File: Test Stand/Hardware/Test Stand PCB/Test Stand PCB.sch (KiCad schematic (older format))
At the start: 18 parts, among them J1 Screw_Terminal_01x02, J2 Screw_Terminal_01x02, J3 Screw_Terminal_01x02, J4 Screw_Terminal_01x04, J5 Screw_Terminal_01x02, U1 AdafruitHuzzah32Breakout, U2 Adafruit_MAX31856, U3 Adafruit_MAX31856, U4 Adafruit_MAX31856, U5 Adafruit_MAX31856, U7 INA_122P, U8 Adafruit_MicroSD_Breakout

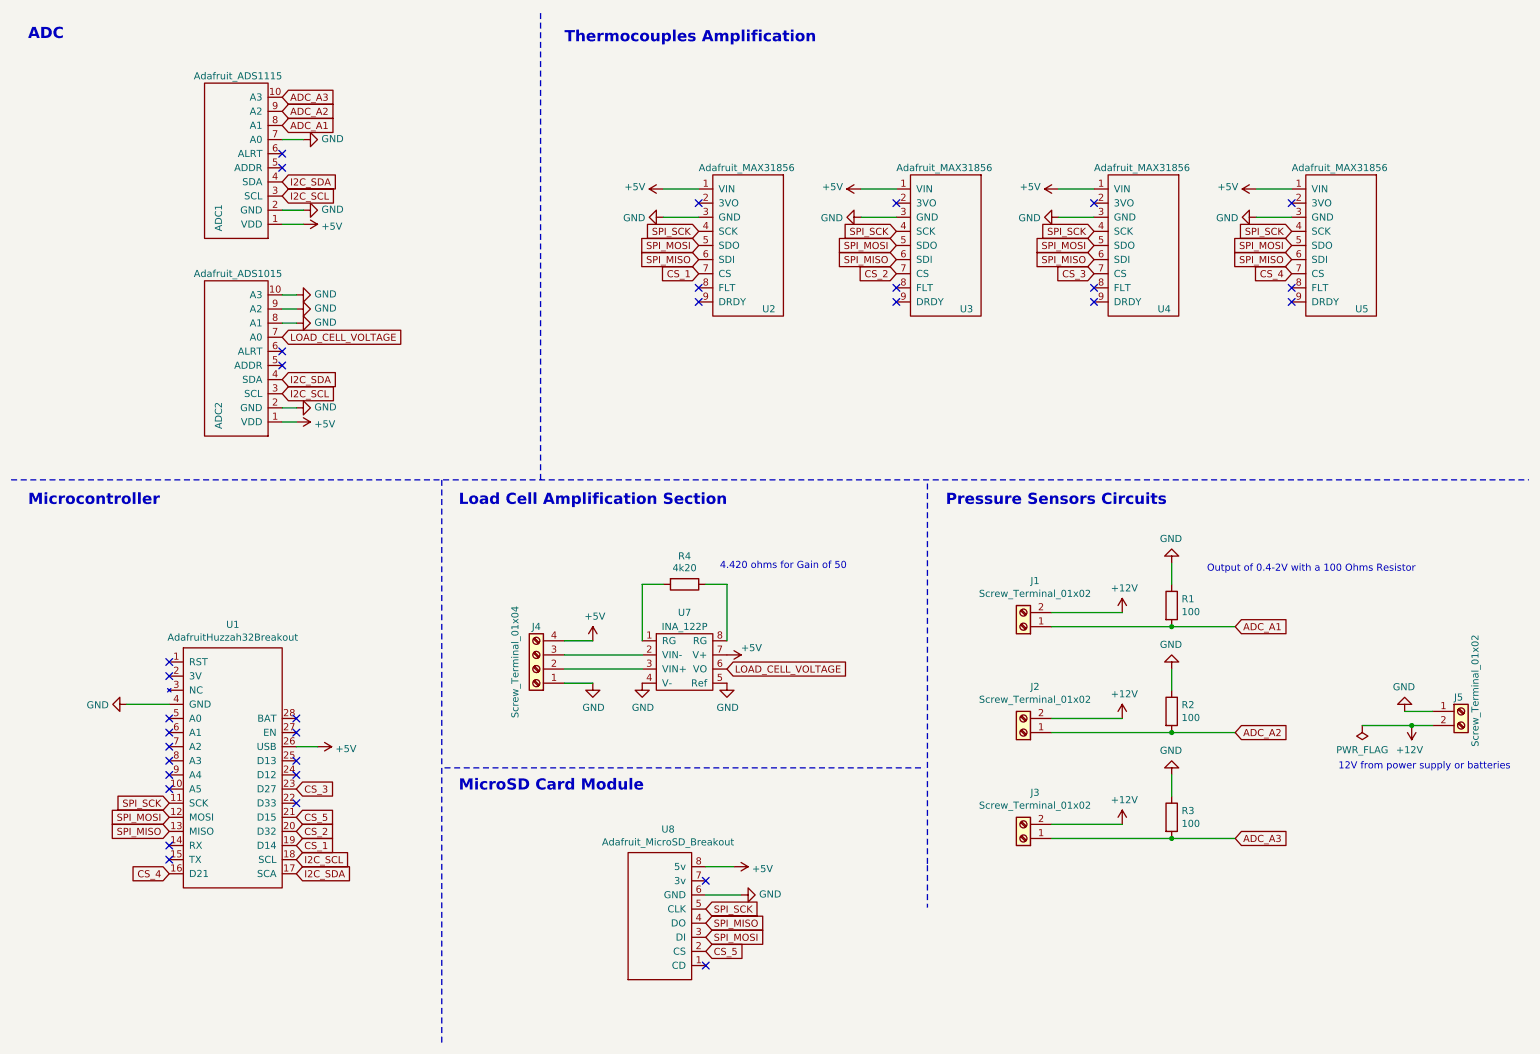
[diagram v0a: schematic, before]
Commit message: Added gerber file for manufacturing of Test Stand PCB v1.0
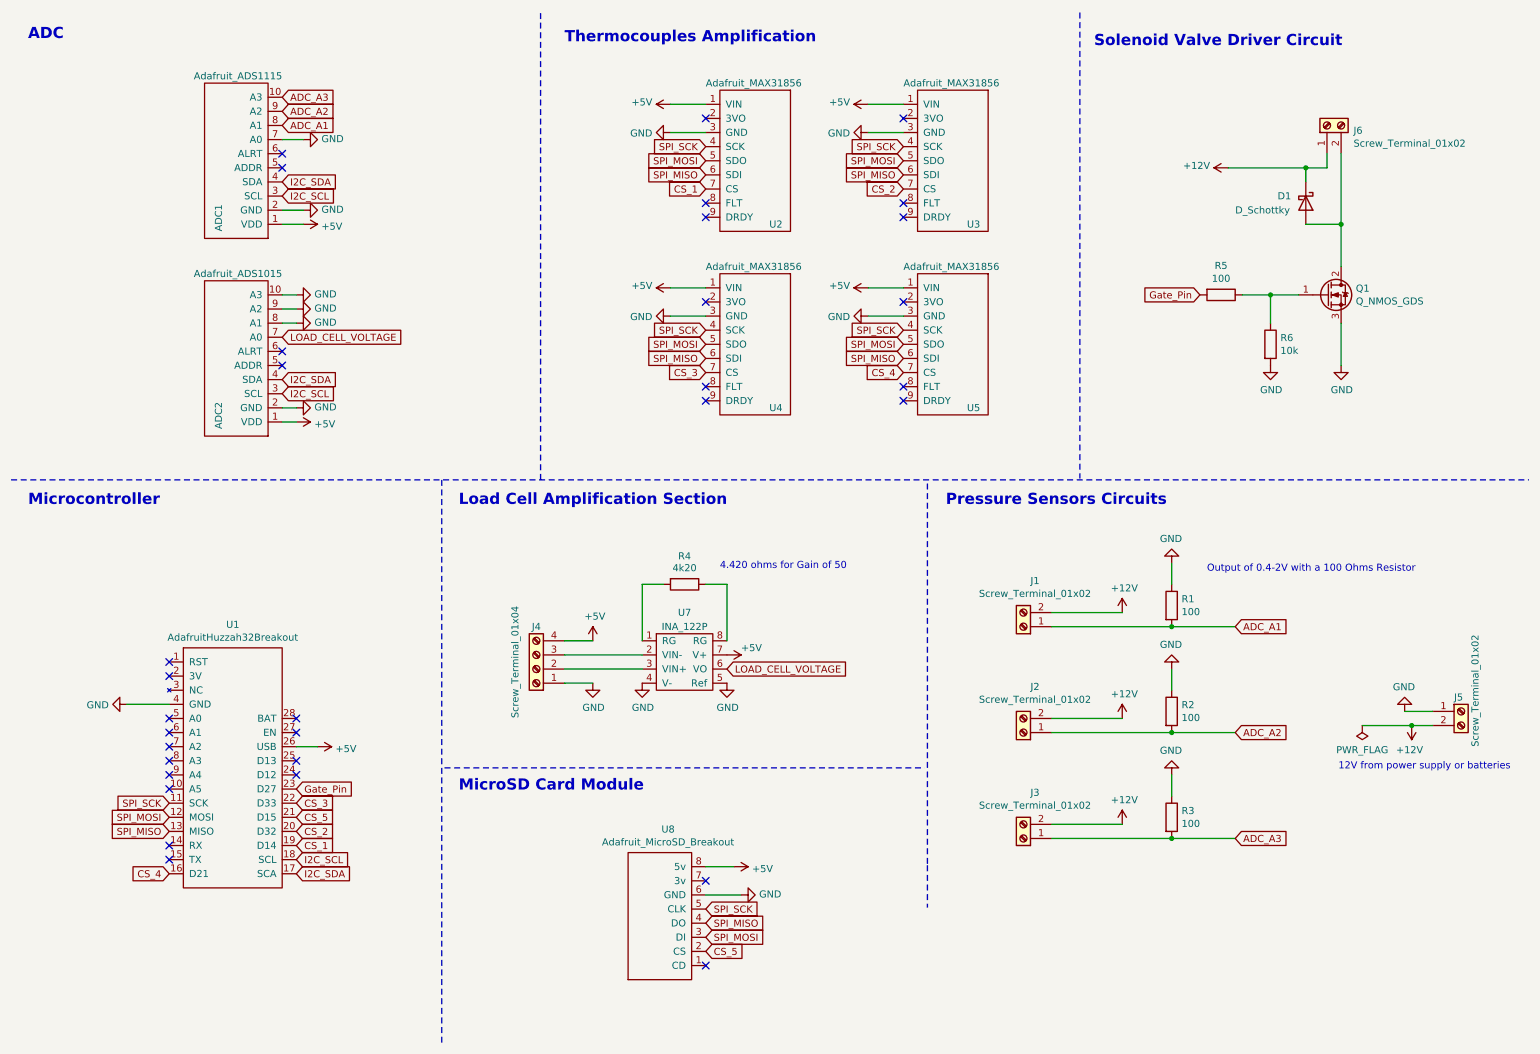
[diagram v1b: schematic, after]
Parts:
- added D1: D_Schottky, Diode_THT:D_DO-41_SOD81_P7.62mm_Horizontal, symbol Device:D_Schottky
- added J6: Screw_Terminal_01x02, TerminalBlock:TerminalBlock_bornier-2_P5.08mm, symbol Connector:Screw_Terminal_01x02
- added Q1: Q_NMOS_GDS, Package_TO_SOT_THT:TO-251-3_Vertical, symbol Device:Q_NMOS_GDS
- added R5: 100, Resistor_THT:R_Axial_DIN0204_L3.6mm_D1.6mm_P5.08mm_Horizontal, symbol Device:R
- added R6: 10k, Resistor_THT:R_Axial_DIN0204_L3.6mm_D1.6mm_P5.08mm_Horizontal, symbol Device:R
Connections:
- net +12V: now also D1.1 (K), J6.1 (Pin_1)
- net CS_3: now also U1.22 (D33); no longer U1.23 (D27)
- net GND: now also Q1.3 (S), R6.2
- new net: Q1.1 (G), R5.1, R6.1
- new net: D1.2 (A), J6.2 (Pin_2), Q1.2 (D)
- new net Gate_Pin: R5.2, U1.23 (D27)
- no-connect marks 33 -> 32
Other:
- note added: "Solenoid Valve Driver Circuit\n"
- moved on the sheet: U2, U3, U4, U5

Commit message: Updated Schematic PDF
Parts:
- ADC1: symbol Test_Stand_Symbol_Library:Adafruit_ADS1115 -> Test-Stand-PCB-rescue:Adafruit_ADS1115-Test_Stand_Symbol_Library
- ADC2: symbol Test_Stand_Symbol_Library:Adafruit_ADS1015 -> Test-Stand-PCB-rescue:Adafruit_ADS1015-Test_Stand_Symbol_Library
- U1: symbol Test_Stand_Symbol_Library:AdafruitHuzzah32Breakout -> Test-Stand-PCB-rescue:AdafruitHuzzah32Breakout-Test_Stand_Symbol_Library
- U2, U3, U4, U5: symbol Test_Stand_Symbol_Library:Adafruit_MAX31856 -> Test-Stand-PCB-rescue:Adafruit_MAX31856-Test_Stand_Symbol_Library
- U7: symbol Test_Stand_Symbol_Library:INA_122P -> Test-Stand-PCB-rescue:INA_122P-Test_Stand_Symbol_Library
- U8: symbol Test_Stand_Symbol_Library:Adafruit_MicroSD_Breakout -> Test-Stand-PCB-rescue:Adafruit_MicroSD_Breakout-Test_Stand_Symbol_Library
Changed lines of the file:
@@
 $EndDescr
 $Comp
-L Test_Stand_Symbol_Library:Adafruit_ADS1115 ADC1
+L Test-Stand-PCB-rescue:Adafruit_ADS1115-Test_Stand_Symbol_Library ADC1
 U 1 1 5F89A5C4
 P 2400 1350
@@
 $EndComp
 $Comp
-L Test_Stand_Symbol_Library:Adafruit_ADS1015 ADC2
+L Test-Stand-PCB-rescue:Adafruit_ADS1015-Test_Stand_Symbol_Library ADC2
 U 1 1 5F89AD1E
 P 2400 2750
@@
 	2500 3400 2400 3400
 $Comp
-L Test_Stand_Symbol_Library:INA_122P U7
+L Test-Stand-PCB-rescue:INA_122P-Test_Stand_Symbol_Library U7
 U 1 1 5F8AD66F
 P 5250 4850
@@
 $EndComp
 $Comp
-L Test_Stand_Symbol_Library:Adafruit_MAX31856 U5
+L Test-Stand-PCB-rescue:Adafruit_MAX31856-Test_Stand_Symbol_Library U5
 U 1 1 5F8AB18D
 P 7150 2850
@@
 $EndComp
 $Comp
-L Test_Stand_Symbol_Library:Adafruit_MAX31856 U3
+L Test-Stand-PCB-rescue:Adafruit_MAX31856-Test_Stand_Symbol_Library U3
 U 1 1 5F8AB175
 P 7150 1550
@@
 $EndComp
 $Comp
-L Test_Stand_Symbol_Library:Adafruit_MAX31856 U4
+L Test-Stand-PCB-rescue:Adafruit_MAX31856-Test_Stand_Symbol_Library U4
 U 1 1 5F8A86F2
 P 5750 2850
@@
 $EndComp
 $Comp
-L Test_Stand_Symbol_Library:Adafruit_MAX31856 U2
+L Test-Stand-PCB-rescue:Adafruit_MAX31856-Test_Stand_Symbol_Library U2
 U 1 1 5F8A1A33
 P 5750 1550
@@
 Load Cell Amplification Section\n
 $Comp
-L Test_Stand_Symbol_Library:Adafruit_MicroSD_Breakout U8
+L Test-Stand-PCB-rescue:Adafruit_MicroSD_Breakout-Test_Stand_Symbol_Library U8
 U 1 1 5F8F764B
 P 5100 6900
@@
 	6970 6540 6970 6840
 $Comp
-L Test_Stand_Symbol_Library:AdafruitHuzzah32Breakout U1
+L Test-Stand-PCB-rescue:AdafruitHuzzah32Breakout-Test_Stand_Symbol_Library U1
 U 1 1 5F7A20EC
 P 2050 5200
